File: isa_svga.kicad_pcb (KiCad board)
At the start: 2 copper layers, 102 x 69.7 mm, 63 parts, among them P1 VGA, U1 TVGA9000i, U2 27C256, U3 256Kx4 70ns, U4 256Kx4 70ns, U5 256Kx4 70ns, U6 256Kx4 70ns, X1 40MHz

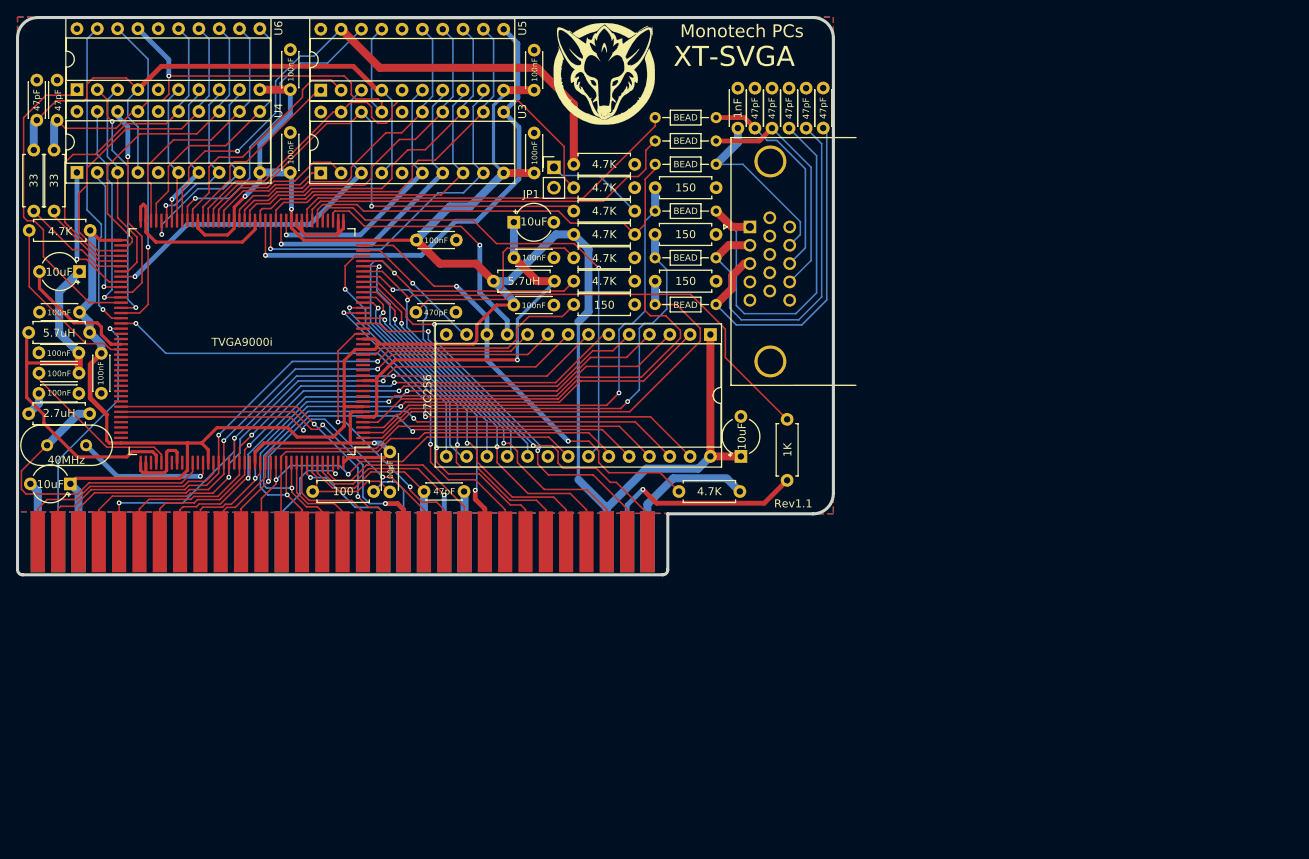
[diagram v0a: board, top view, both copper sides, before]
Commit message: Add files via upload
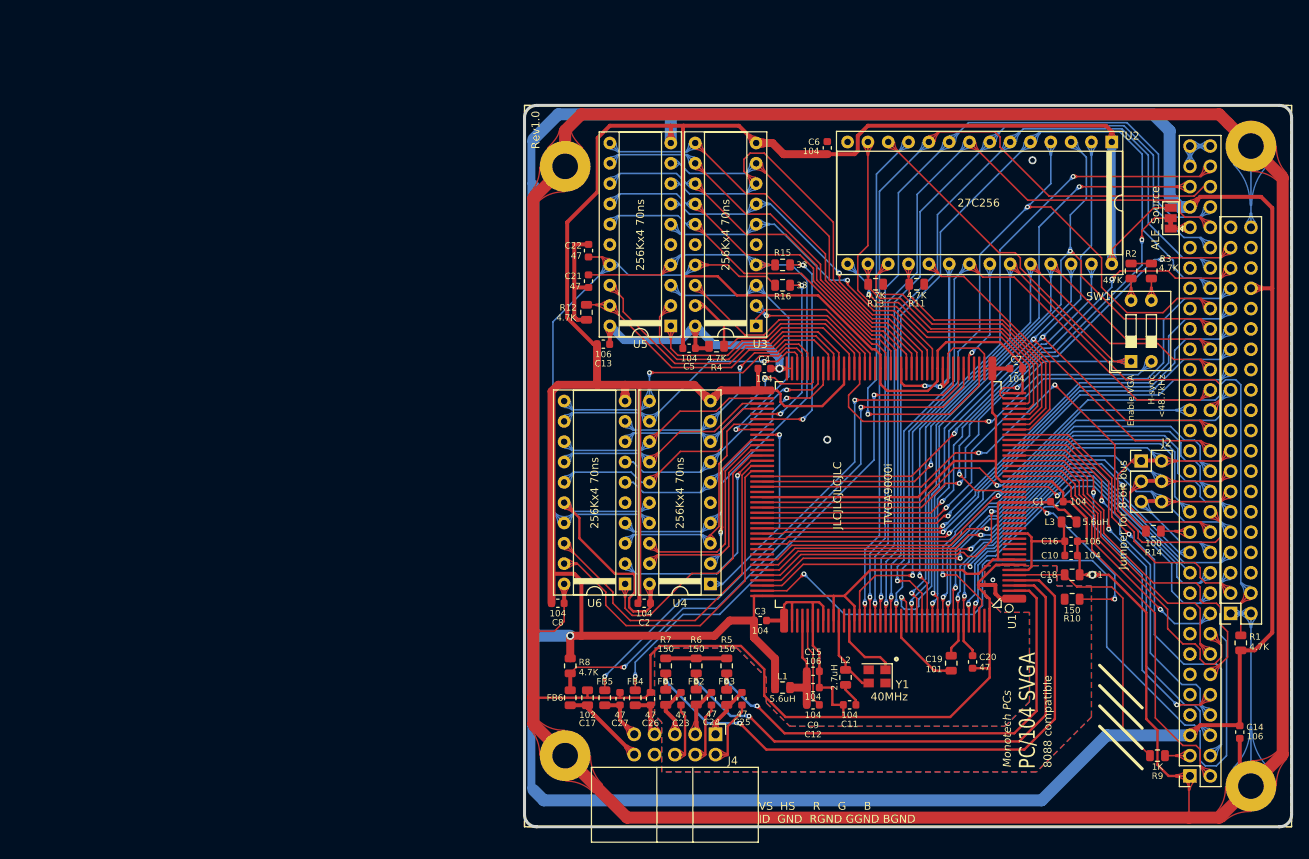
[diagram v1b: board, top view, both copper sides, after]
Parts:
- removed BUS1: BUSPC_DEV, Custom:Conn_Bus_ISA8_TVGA
- removed G***: LOGO, Custom:Monotech_Logo_150
- removed JP1: HSYNC_SEL, Connector_PinHeader_2.54mm:PinHeader_1x02_P2.54mm_Vertical
- removed P1: VGA, Custom:DSUB-15-HD_Female_Horizontal_CONNFLY_DS1308
- removed X1: 40MHz, Crystal:Crystal_HC49-4H_Vertical
- added J1: PC104, Custom:PC104_Platform, F.Cu at (260.9, 166.1)
- added J2: Jumper for 8-bit bus, Custom:Triple-bridged-jumper, F.Cu at (242.1, 120.4)
- added J3: PC104_16, Connector_PinSocket_2.54mm:PinSocket_2x20_P2.54mm_Vertical, F.Cu at (253.2, 139.4)
- added J4: VGA Output, Connector_IDC:IDC-Header_2x05_P2.54mm_Horizontal, F.Cu at (188.8, 154.6)
- added JP4: ALE_Source, Jumper:SolderJumper-3_P1.3mm_Bridged12_Pad1.0x1.5mm, F.Cu at (245.7, 90.0)
- added NT7: NetTie, NetTie:NetTie-2_SMD_Pad0.5mm, F.Cu at (222.2, 135.9)
- added SW1: VGA Config, Button_Switch_THT:SW_DIP_SPSTx02_Slide_9.78x7.26mm_W7.62mm_P2.54mm, F.Cu at (240.8, 108.0)
- added Y1: 40MHz, Oscillator:Oscillator_SMD_Abracon_ASE-4Pin_3.2x2.5mm, F.Cu at (209.0, 147.3)
- C1, C10, C11, C12, C2, C3, C4, C5, C6, C7, C8, C9: value 100nF -> 104; footprint Capacitor_THT:C_Disc_D4.3mm_W1.9mm_P5.00mm -> Custom KiCad Library:C_0603_1608Metric
- C13, C14, C15, C16: value 10uF -> 106; footprint Capacitor_THT:CP_Radial_Tantal_D4.5mm_P5.00mm -> Custom KiCad Library:C_0603_1608Metric
- C17: value 1nF -> 102; footprint Capacitor_THT:C_Disc_D4.3mm_W1.9mm_P5.00mm -> Custom KiCad Library:C_0805_2012Metric
- C18: value 470pF -> 471; footprint Capacitor_THT:C_Disc_D4.3mm_W1.9mm_P5.00mm -> Custom KiCad Library:C_0805_2012Metric
- C19: value 100pF -> 101; footprint Capacitor_THT:C_Disc_D4.3mm_W1.9mm_P5.00mm -> Custom KiCad Library:C_0805_2012Metric
- C20, C21, C22, C23, C24, C25, C26, C27: value 47pF -> 47; footprint Capacitor_THT:C_Disc_D4.3mm_W1.9mm_P5.00mm -> Custom KiCad Library:C_0603_1608Metric
- FB1, FB2, FB3, FB4, FB5, FB6: footprint Resistor_THT:R_Axial_DIN0204_L3.6mm_D1.6mm_P7.62mm_Horizontal -> Custom KiCad Library:C_0805_2012Metric
- L1, L3: value 5.7uH -> 5.6uH; footprint Resistor_THT:R_Axial_DIN0207_L6.3mm_D2.5mm_P7.62mm_Horizontal -> Custom KiCad Library:C_0805_2012Metric
- L2: footprint Resistor_THT:R_Axial_DIN0207_L6.3mm_D2.5mm_P7.62mm_Horizontal -> Custom KiCad Library:C_0805_2012Metric
- R1, R10, R14, R15, R16, R2, R3, R4, R8, R9: footprint Resistor_THT:R_Axial_DIN0207_L6.3mm_D2.5mm_P7.62mm_Horizontal -> Custom KiCad Library:R_0805_2012Metric
- R11, R12, R13: value 150 -> 4.7K; footprint Resistor_THT:R_Axial_DIN0207_L6.3mm_D2.5mm_P7.62mm_Horizontal -> Custom KiCad Library:R_0805_2012Metric
- R5, R6, R7: value 4.7K -> 150; footprint Resistor_THT:R_Axial_DIN0207_L6.3mm_D2.5mm_P7.62mm_Horizontal -> Custom KiCad Library:R_0805_2012Metric
- U1: footprint Custom:PQFP-160_28x28mm_P0.65mm -> Custom KiCad Library:PQFP-160_28x28mm_P0.65mm_LongPads
- U2: footprint Package_DIP:DIP-28_W15.24mm_Socket -> Custom KiCad Library:DIP-28_W15.24mm_Socket
- U3, U4, U5, U6: footprint Package_DIP:DIP-20_W7.62mm_Socket -> Custom KiCad Library:DIP-20_W7.62mm_Socket
- moved R1 160.0 mm to (254.5, 143.1), turned to 270 degrees
- moved C7 114.4 mm to (226.4, 108.8), turned to 180 degrees
- moved C11 108.6 mm to (205.6, 150.9), turned to 180 degrees
- moved L2 107.3 mm to (205.1, 147.4), turned to 90 degrees
- moved C15 104.4 mm to (201.0, 146.7), turned to 0 degrees
- moved C9 100.9 mm to (201.0, 148.7), turned to 0 degrees
- moved C12 100.7 mm to (201.0, 150.9), turned to 0 degrees
- moved R14 97.6 mm to (243.6, 129.2)
- moved L1 97.3 mm to (197.2, 148.7), turned to 0 degrees
- moved U4 94.4 mm to (188.2, 135.8), turned to 180 degrees
- moved R15 93.8 mm to (197.2, 95.9), turned to 180 degrees
- moved U6 92.3 mm to (177.5, 135.8), turned to 180 degrees
- moved R16 91.5 mm to (197.2, 98.4), turned to 180 degrees
- moved C18 88.4 mm to (233.4, 134.6)
- moved C1 86.5 mm to (231.5, 125.5)
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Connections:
- net /AVDD1 renamed /SYNC_VDD
- net /AVDD2 renamed /DAC_VDD
- net Net-(R1-Pad1) renamed /~MEMCS16
- C17 pad 1: Net-(C17-Pad1) -> GND
- C17 pad 2: GND -> /xMONITOR
- C23 pad 1: /RED -> /DAC_GND
- C23 pad 2: GND -> /xRED
- C24 pad 1: /GREEN -> /DAC_GND
- C24 pad 2: GND -> /xGREEN
- C25 pad 1: /BLUE -> /DAC_GND
- C25 pad 2: GND -> /xBLUE
- C26 pad 1: Net-(C26-Pad1) -> GND
- C26 pad 2: GND -> /xHSYNC
- C27 pad 1: Net-(C27-Pad1) -> GND
- C27 pad 2: GND -> /xVSYNC
- FB1 pad 2: /RED -> /xRED
- FB2 pad 2: /GREEN -> /xGREEN
- FB3 pad 2: /BLUE -> /xBLUE
- FB4 pad 1: Net-(C26-Pad1) -> /HSYNC
- FB4 pad 2: /HSYNC -> /xHSYNC
- FB5 pad 1: Net-(C27-Pad1) -> /VSYNC
- FB5 pad 2: /VSYNC -> /xVSYNC
- FB6 pad 1: Net-(C17-Pad1) -> /MONITOR
- FB6 pad 2: /MONITOR -> /xMONITOR
- R10 pad 2: GND -> /DAC_GND
- R11 pad 1: /R -> /RMD6
- R12 pad 1: /G -> /MD7
- R13 pad 1: /B -> /RMD4
- R2 pad 1: /MD7 -> Net-(R2-Pad1)
- R3 pad 1: /RMD6 -> Net-(R3-Pad1)
- R4 pad 1: /RMD4 -> /MD3
- R5 pad 1: /RMD1 -> /B
- R5 pad 2: GND -> /DAC_GND
- R6 pad 1: /MD2 -> /G
- R6 pad 2: Net-(JP1-Pad1) -> /DAC_GND
- R7 pad 1: /MD3 -> /R
- R7 pad 2: GND -> /DAC_GND
- U1 pad 1: GND -> /DAC_GND
- U1 pad 10: Net-(U1-Pad10) -> (no net)
- U1 pad 100: Net-(U1-Pad100) -> (no net)
- U1 pad 103: Net-(U1-Pad103) -> /D15
- U1 pad 104: Net-(U1-Pad104) -> /D14
- U1 pad 105: Net-(U1-Pad105) -> /D13
- U1 pad 106: Net-(U1-Pad106) -> /D12
- U1 pad 107: Net-(U1-Pad107) -> /D11
- U1 pad 108: Net-(U1-Pad108) -> /D10
- U1 pad 109: Net-(U1-Pad109) -> /D9
- U1 pad 11: Net-(U1-Pad11) -> (no net)
- U1 pad 110: Net-(U1-Pad110) -> /D8
- U1 pad 111: Net-(U1-Pad111) -> (no net)
- U1 pad 112: Net-(U1-Pad112) -> (no net)
- U1 pad 113: /A17 -> /LA17
- U1 pad 114: /A18 -> /LA18
- U1 pad 115: /A19 -> /LA19
- U1 pad 116: Net-(U1-Pad116) -> /LA20
- U1 pad 117: Net-(U1-Pad117) -> /LA21
- U1 pad 118: Net-(U1-Pad118) -> /LA22
- U1 pad 119: Net-(U1-Pad119) -> /LA23
- U1 pad 12: Net-(U1-Pad12) -> (no net)
- U1 pad 123: Net-(U1-Pad123) -> (no net)
- U1 pad 127: Net-(U1-Pad127) -> (no net)
- U1 pad 129: Net-(U1-Pad129) -> (no net)
- U1 pad 132: Net-(U1-Pad132) -> (no net)
- U1 pad 14: Net-(U1-Pad14) -> (no net)
- U1 pad 15: Net-(U1-Pad15) -> (no net)
- U1 pad 159: Net-(U1-Pad159) -> (no net)
- U1 pad 16: Net-(U1-Pad16) -> (no net)
- U1 pad 17: Net-(U1-Pad17) -> (no net)
- U1 pad 20: Net-(U1-Pad20) -> (no net)
- U1 pad 21: VCC -> Net-(JP4-Pad2)
- U1 pad 44: Net-(U1-Pad44) -> (no net)
- U1 pad 63: Net-(U1-Pad63) -> (no net)
- U1 pad 9: Net-(U1-Pad9) -> (no net)
- U1 pad 99: Net-(U1-Pad99) -> /~SBHE
- U3 pad 5: Net-(U3-Pad5) -> (no net)
- U4 pad 5: Net-(U4-Pad5) -> (no net)
- U5 pad 5: Net-(U5-Pad5) -> (no net)
- U6 pad 5: Net-(U6-Pad5) -> (no net)
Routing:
- net GND: track 122.5 -> 767.3 mm, vias 1 -> 6
- net VCC: track 327.9 -> 794.0 mm, vias 2 -> 1
- net /LA23: track 0.00 -> 109.1 mm, vias 0 -> 1
- net /~SBHE: track 0.00 -> 81.0 mm, vias 0 -> 2
- net /~MEMCS16: track 21.8 -> 101.3 mm, vias 0 -> 1
- net /D14: track 0.00 -> 76.5 mm, vias 0 -> 2
- net /D13: track 0.00 -> 75.9 mm, vias 0 -> 1
- net /D15: track 0.00 -> 75.3 mm, vias 0 -> 2
- net /LA21: track 0.00 -> 74.9 mm, vias 0 -> 1
- net /LA20: track 0.00 -> 74.8 mm, vias 0 -> 1
- net Net-(C18-Pad1): track 108.4 -> 35.9 mm
- net /D12: track 0.00 -> 71.8 mm, vias 0 -> 1
- net /D11: track 0.00 -> 70.1 mm, vias 0 -> 1
- net /LA22: track 0.00 -> 70.0 mm, vias 0 -> 1
- net /D10: track 0.00 -> 68.4 mm, vias 0 -> 1
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- added copper zone on B.Cu, net /DAC_GND
- added copper zone on F.Cu, net /DAC_GND
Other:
- board size 102 x 69.7 mm -> 95.9 x 90.2 mm
- net class Default: clearance 0.2 -> 0.17
- net class Power removed
- rule trace_clearance: 0.2 -> 0.17
- board text added: "8088 compatible"
- board text added: "Enable VGA H-sync <48.7kHz"
- board text added: "JLCJLCJLCJLC"
- board text added: "PC/104 SVGA"
- board text added: "Rev1.0"
- board text added: "VS HS R G B ID GND RGND GGND BGND"
- board text removed: "Close JP1 for monitor H-Sync < 48.7 kHz"
- board text removed: "Rev1.1"
- board text removed: "Use 256Ki x 4bit 70ns DIP-20 DRAM ICs for VRAM. Such as MT4C4256, TC514256, MCM514256. For 256KiB VRAM, populate U3 and U4. For 512KiB VRAM, populate all four sockets."
- board text removed: "XT-SVGA"
